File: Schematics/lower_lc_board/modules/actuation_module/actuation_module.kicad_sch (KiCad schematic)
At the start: 7 parts

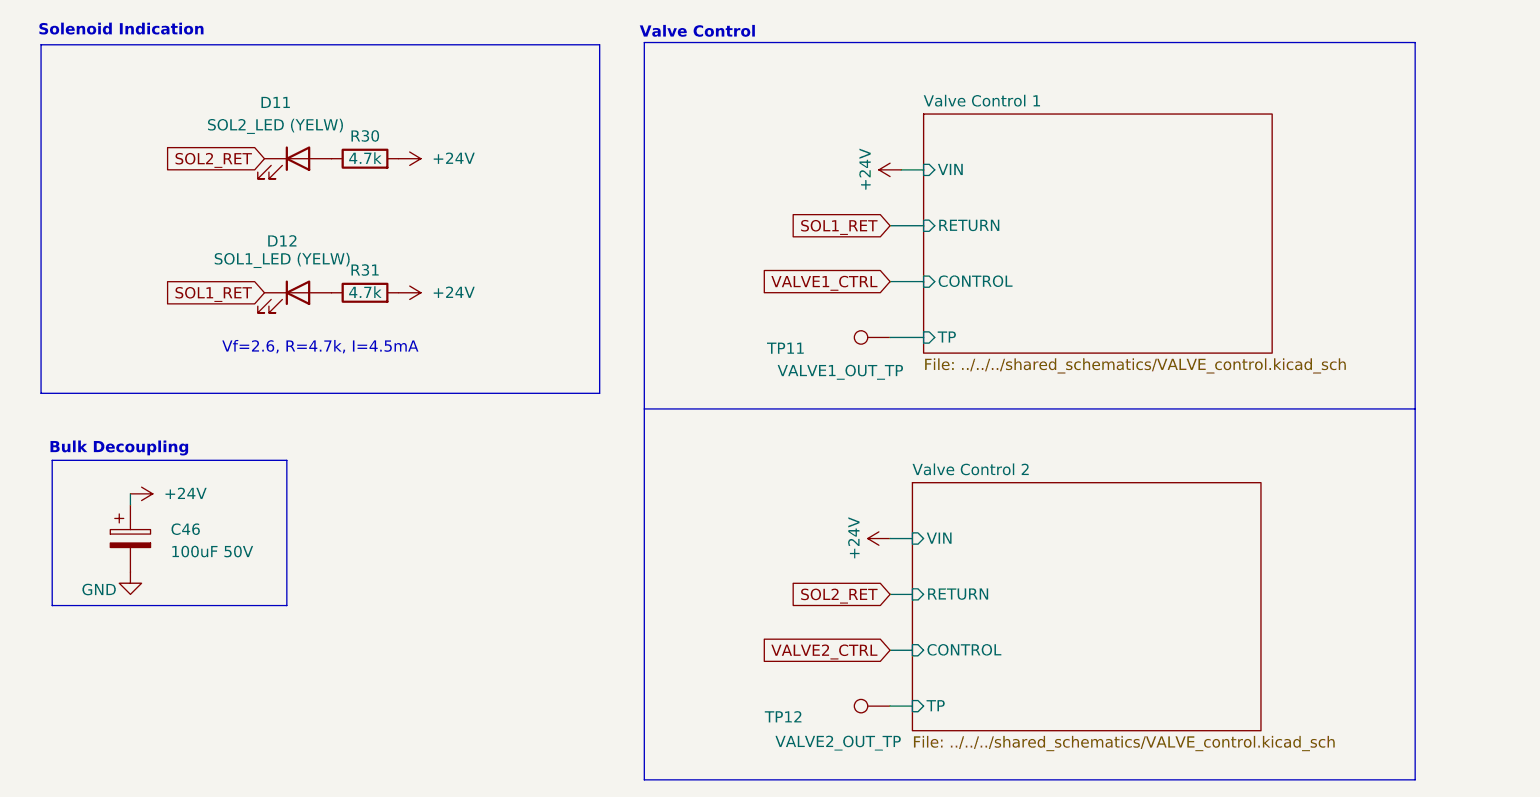
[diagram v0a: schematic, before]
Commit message: organizational work
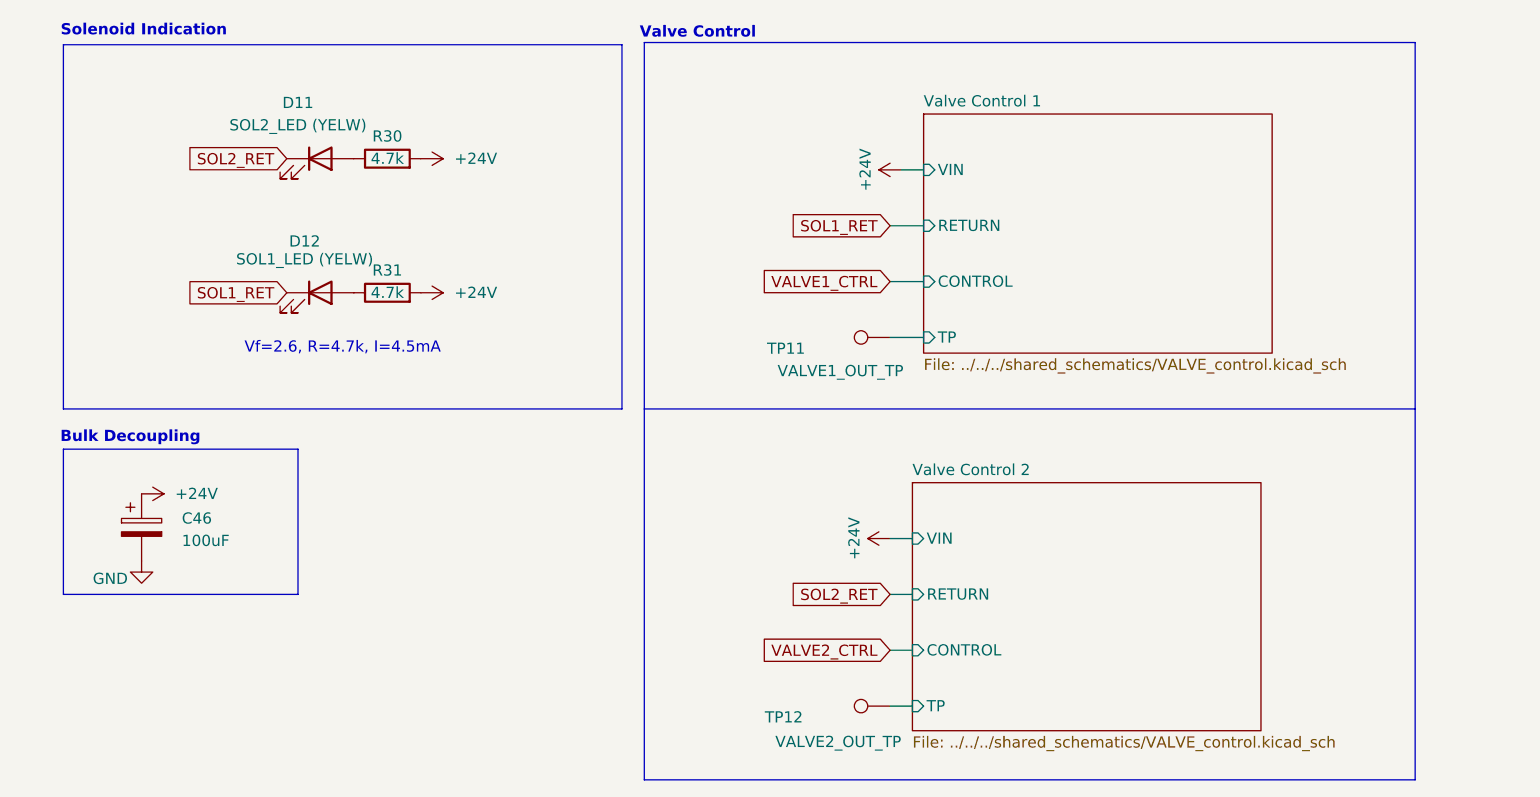
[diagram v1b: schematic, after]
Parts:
- C46: value 100uF 50V -> 100uF
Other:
- moved on the sheet: C46, D11, D12, R30, R31
